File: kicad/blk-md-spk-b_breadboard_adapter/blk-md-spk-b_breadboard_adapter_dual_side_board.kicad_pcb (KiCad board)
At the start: 2 copper layers, 24.6 x 34.2 mm, 4 parts, among them J1 SCJ-0354-5PU, P1 CONNECTOR, P2 CONNECTOR, U1 BLK-MD-SPK-B

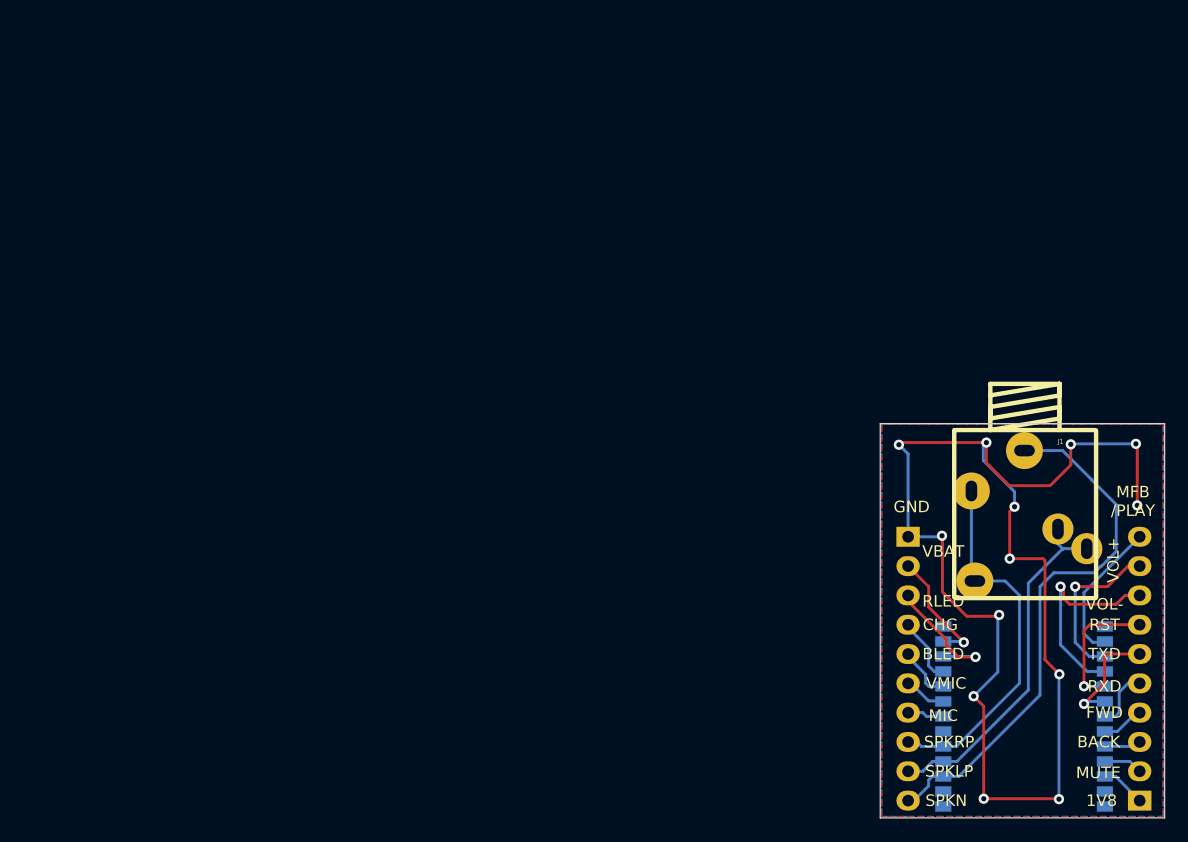
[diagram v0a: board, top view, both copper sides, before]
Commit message: updated version
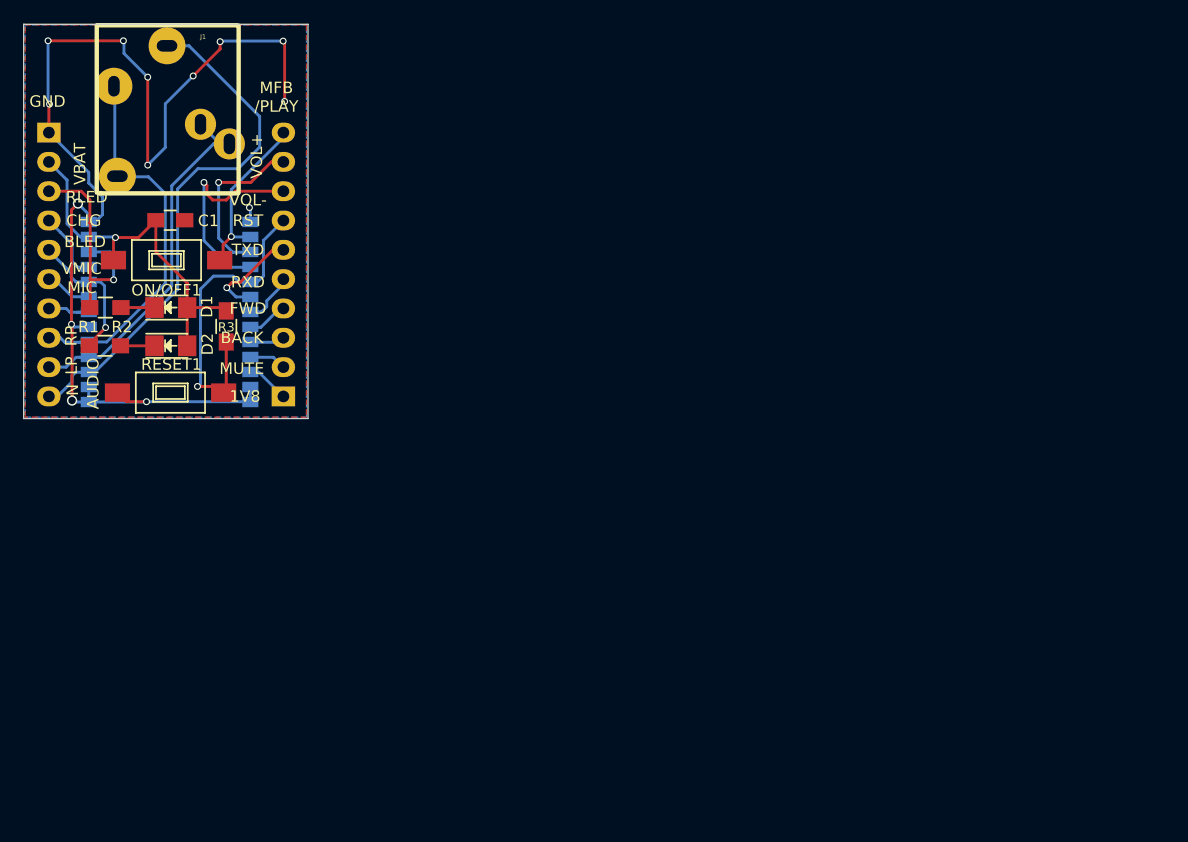
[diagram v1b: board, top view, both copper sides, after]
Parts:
- added C1: 100n, Capacitors_SMD:C_0805_HandSoldering, F.Cu at (122.2, 113.4)
- added D1: LED, LEDs:LED-1206, F.Cu at (122.3, 121.0)
- added D2: LED, LEDs:LED-1206, F.Cu at (122.3, 124.3)
- added ON/OFF1: SW_PUSH, Buttons_Switches_SMD:SW_SPST_FSMSM, F.Cu at (121.9, 116.9)
- added R1: 470, Resistors_SMD:R_0805_HandSoldering, F.Cu at (116.6, 121.0)
- added R2: 470, Resistors_SMD:R_0805_HandSoldering, F.Cu at (116.6, 124.3)
- added R3: 10k, Resistors_SMD:R_0805_HandSoldering, F.Cu at (127.1, 122.6)
- added RESET1: SW_PUSH, Buttons_Switches_SMD:SW_SPST_FSMSM, F.Cu at (122.3, 128.4)
- J1: value SCJ-0354-5PU -> SCJ368R1NUS0B00G; footprint jacks:SCJ-0354-5PU -> jacks:SCJ-0354-5PU_no_screew
- U1: footprint my_modules:BLK-MD-SPK-B -> my_modules:BLK-MD-SPK-B_no_up_silk
- moved P2 87.8 mm to (111.7, 105.8), turned to 180 degrees
- moved J1 82.2 mm to (122.0, 96.6)
- moved U1 81.9 mm to (113.9, 135.5)
- moved P1 77.9 mm to (132.1, 128.7), turned to 0 degrees
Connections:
- U1 pad 14: (no net) -> GND
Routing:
- net Net-(C1-Pad1): track 11.8 -> 33.1 mm
- net Net-(P1-Pad7): track 11.7 -> 28.5 mm
- net GND: track 112.7 -> 103.9 mm, vias 13 -> 14
- net Net-(P2-Pad3): track 13.0 -> 20.1 mm
- net Net-(P2-Pad5): track 5.44 -> 12.2 mm, vias 0 -> 1
- net Net-(D2-Pad1): track 0.00 -> 2.95 mm
- net Net-(D1-Pad1): track 0.00 -> 2.91 mm
- net Net-(ON/OFF1-Pad1): track 12.5 -> 15.0 mm, vias 0 -> 1
- net Net-(J1-Pad1): track 48.1 -> 46.8 mm
- net Net-(P1-Pad6): track 9.85 -> 8.64 mm
- net Net-(P1-Pad5): track 5.25 -> 4.59 mm
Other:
- net class Default: clearance 0.254 -> 0.2; trace_width 0.254 -> 0.25; via_dia 0.889 -> 0.6; via_drill 0.635 -> 0.4
- rule pad_to_mask_clearance: 0 -> 0.2
- rule trace_clearance: 0.254 -> 0.2
- rule trace_min: 0.254 -> 0.2
- rule via_min_drill: 0.508 -> 0.3
- rule via_min_size: 0.889 -> 0.4
- board text added: "AUDIO"
- board text added: "LP"
- board text added: "N"
- board text added: "RP"
- board text removed: "SPKLP"
- board text removed: "SPKN"
- board text removed: "SPKRP"
